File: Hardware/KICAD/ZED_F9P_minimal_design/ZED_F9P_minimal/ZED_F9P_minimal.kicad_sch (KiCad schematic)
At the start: 15 parts, among them IC1 ZED-F9P-15B, J1 Conn_Coaxial_Small

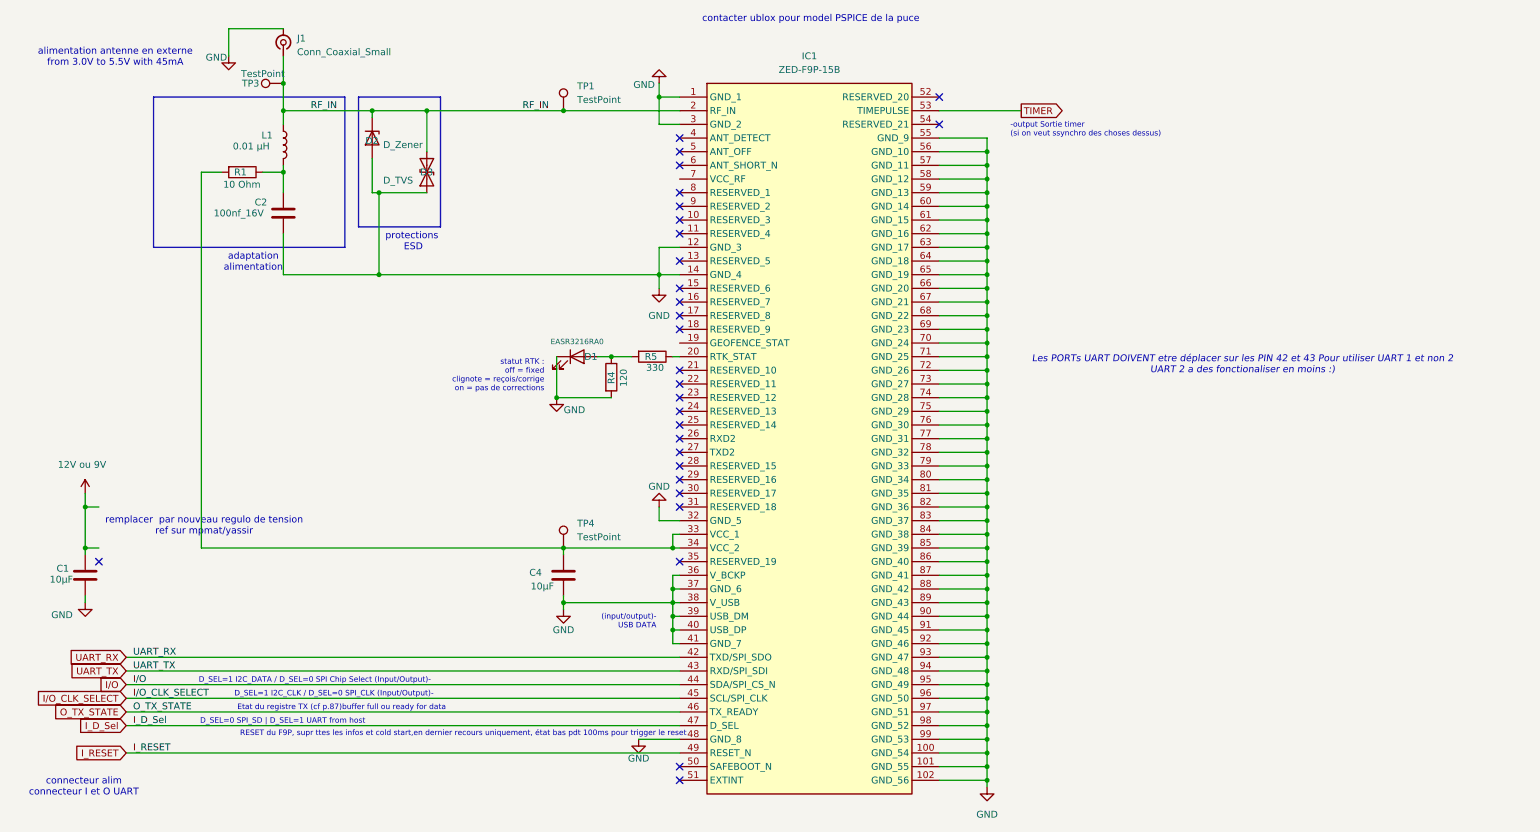
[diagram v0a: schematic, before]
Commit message: finalised first iteration of schematic
schematic 1.0,, gonna start pcb rooting
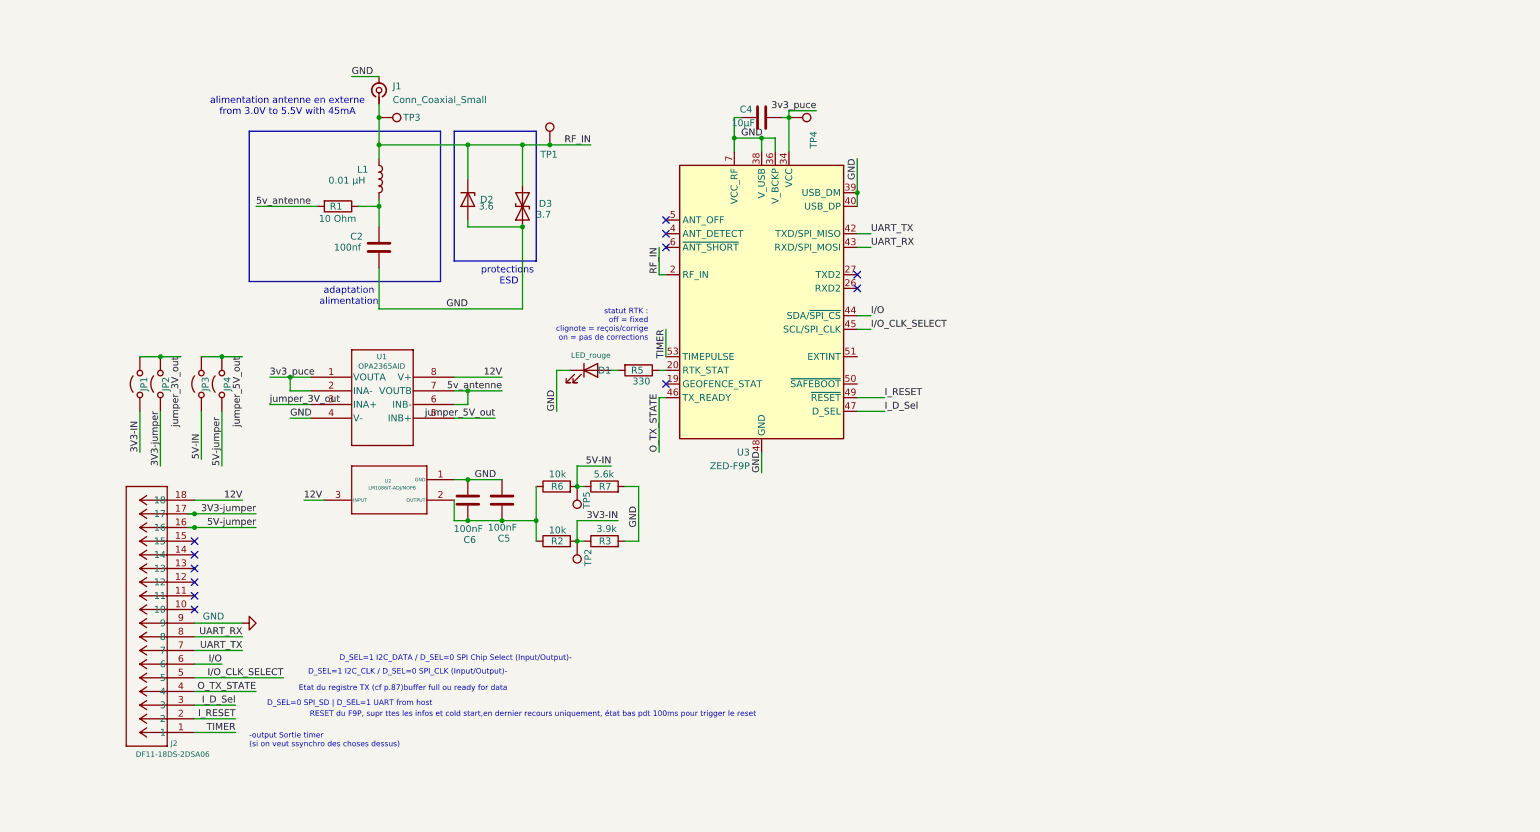
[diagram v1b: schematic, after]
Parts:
- removed C1: 10µF, 1uF:YAG_CC0603_YAG, symbol Device:C
- removed IC1: ZED-F9P-15B, RF_GPS:ublox_ZED, symbol ZED-F9P-15B:ZED-F9P-15B
- removed R4: 120, 120ohm:RC0805N_YAG, symbol Device:R
- added C5, C6: 100nF, Capacitor_SMD:C_0805_2012Metric, symbol Device:C
- added J2: DF11-18DS-2DSA06, Connector:CON18_2X9_U_DF11_HIR, symbol CON2x09:DF11-18DS-2DSA06
- added JP1, JP2, JP3, JP4: Jumper_2_Open, Connector:CON_1x02, symbol Jumper:Jumper_2_Open
- added R2, R6: 10k, res_SMD_10kohm:YAG_R0805_YAG, symbol Device:R
- added R3: 3.9k, res_SMD_4.3kohm:RC0805N_YAG, symbol Device:R
- added R7: 5.6k, res_SMD_5.6kohm:RC0805N_YAG, symbol Device:R
- added TP2, TP5: TestPoint, TestPoint:CONN1_5011_KEY, symbol Connector:TestPoint
- added U1: OPA2365AID, 00_OPA2365:D8, symbol OPA2365:OPA2365AID
- added U2: LM1086IT-ADJ/NOPB, LM1086:NDE0003B, symbol LM1086:LM1086IT-ADJ_NOPB
- added U3: ZED-F9P, RF_GPS:ublox_ZED, symbol RF_GPS:ZED-F9P
- C2: value 100nf_16V -> 100nf; footprint 0_1uF:YAG_CC0603_YAG -> Capacitor_SMD:C_0805_2012Metric
- C4: footprint 1uF:YAG_CC0603_YAG -> Capacitor_SMD:C_0805_2012Metric
- D1: value EASR3216RA0 -> LED_rouge; footprint (none) -> LED_SMD:LED_0805_2012Metric
- D2: value D_Zener -> 3.6; footprint (none) -> Diode_SMD:Zener_3.6V
- D3: value D_TVS -> 3.7; footprint (none) -> Diode_SMD:D_SOD962_TVS_3.7V
- L1: footprint 0_01uH:STA_RMCF1206_STP -> Inductor_SMD:L_0805_2012Metric
- R1: footprint 10_Ohm:RC0402N_YAG -> res_SMD_330ohm:RC0805N_YAG
- R5: footprint 330_ohm:RC0603N_YAG -> res_SMD_330ohm:RC0805N_YAG
- TP1, TP3, TP4: footprint (none) -> TestPoint:CONN1_5011_KEY
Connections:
- net GND: now also C5.2, C6.2, J2.9, R3.2, R7.2, U1.4 (V-), U2.1 (GND), U3.1 (GND), U3.12 (GND), U3.14 (GND), U3.3 (GND), U3.32 (GND), U3.36 (V_BCKP), U3.37 (GND), U3.38 (V_USB), U3.39 (USB_DM), U3.40 (USB_DP), U3.41 (GND), U3.48 (GND), U3.55 (GND), U3.7 (VCC_RF)
- net I_D_Sel: now also J2.3, U3.47 (D_SEL)
- net I_RESET: now also J2.2, U3.49 (~{RESET})
- net I/O : now also J2.6, U3.44 (SDA/~{SPI_CS})
- net I/O_CLK_SELECT: now also J2.5, U3.45 (SCL/SPI_CLK)
- net O_TX_STATE: now also J2.4, U3.46 (TX_READY)
- net RF_IN: now also U3.2 (RF_IN)
- net TIMER: now also J2.1, U3.53 (TIMEPULSE)
- net UART_RX: now also J2.8, U3.43 (RXD/SPI_MOSI)
- net UART_TX: now also J2.7, U3.42 (TXD/SPI_MISO)
- net 3v3_puce: now reaches C4.1, TP4.1
- net 3v3_puce: now also U1.1 (VOUTA), U1.2 (INA-), U3.33 (VCC), U3.34 (VCC); no longer R1.2
- net at R5.1: now also U3.20 (RTK_STAT)
- new net: C5.1, C6.1, R2.1, R6.1, U2.2 (OUTPUT)
- new net 12V: J2.18, U1.8 (V+), U2.3 (INPUT)
- new net 3V3-IN: JP1.1 (A), R2.2, R3.1, TP2.1
- new net 3V3-jumper: J2.17, JP2.1 (A)
- new net 5V-IN: JP3.1 (A), R6.2, R7.1, TP5.1
- new net 5V-jumper: J2.16, JP4.1 (A)
- new net 5v_antenne: R1.2, U1.6 (INB-), U1.7 (VOUTB)
- new net jumper_3V_out: JP1.2 (B), JP2.2 (B), U1.3 (INA+)
- new net jumper_5V_out: JP3.2 (B), JP4.2 (B), U1.5 (INB+)
- no-connect marks 29 -> 12
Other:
- note removed: "(input/output)- USB DATA"
- note removed: "Les PORTs UART DOIVENT etre déplacer sur les PIN 42 et 43 Pour utiliser UART 1 et non 2 UART 2 a des fonctionaliser en moins :)"
- note removed: "connecteur alim connecteur I et O UART"
- note removed: "contacter ublox pour model PSPICE de la puce"
- note removed: "remplacer par nouveau regulo de tension ref sur mpmat/yassir"
- moved on the sheet: C2, C4, D1, D2, D3, J1, L1, R1, R5, TP1, TP3, TP4
